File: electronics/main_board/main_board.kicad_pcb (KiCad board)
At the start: 6 copper layers, 50 x 47 mm, 95 parts, among them CN1 DB141R-2.54-2P, CN3 KF202-5.0-3P, U1 HUSB238A-BB001-QN16R, U10 TJA1051TK/3, U11 NTTFS5C454NL, U13 NTTFS5C454NL, U14 NTTFS5C454NL, U15 NTTFS5C454NL, U16 NTTFS5C454NL, U17 NTTFS5C454NL, U18 TJA1051TK/3, U2 LMR51420YDD, U3 TPS62933DRL, U6 ESP32-S3-WROOM-1, U7 STM32G474VEH6, U8 DRV8323SRTA, U9 AFD01-S35FCA-00

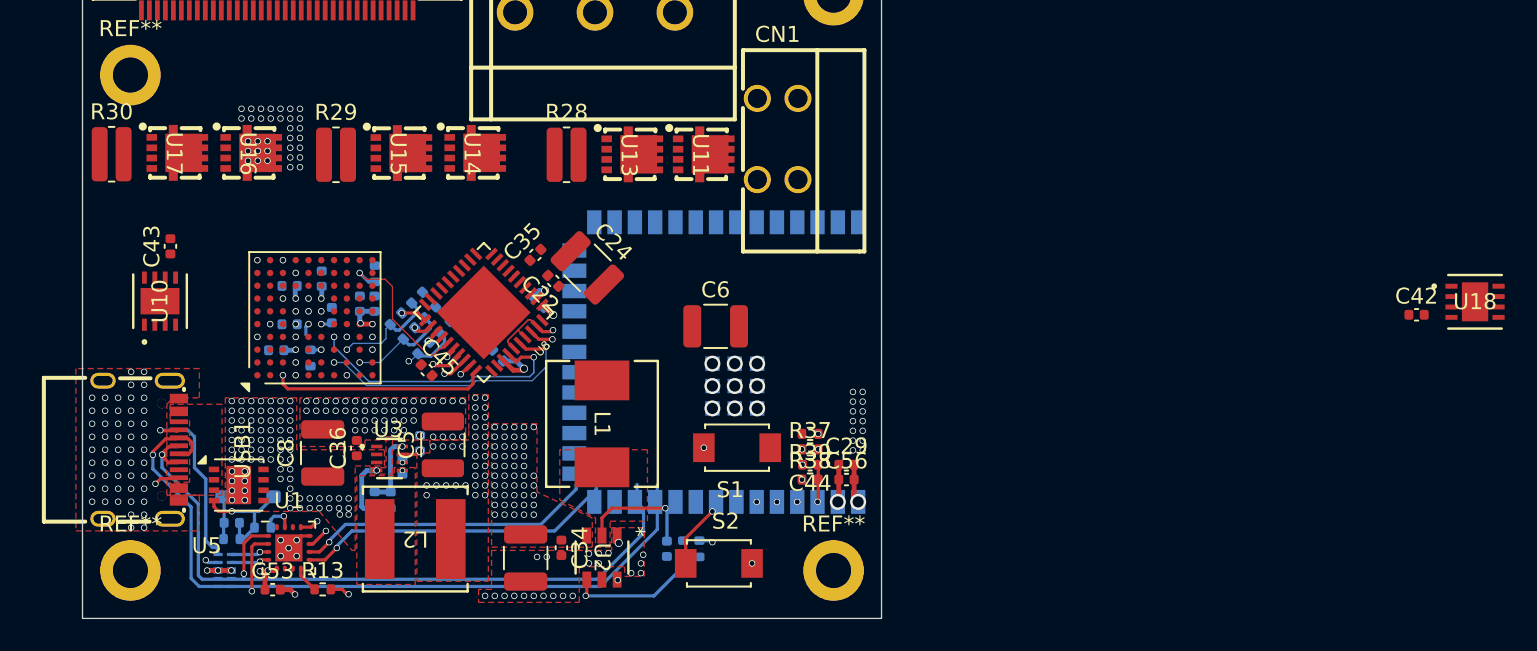
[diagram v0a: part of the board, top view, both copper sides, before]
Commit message: fix
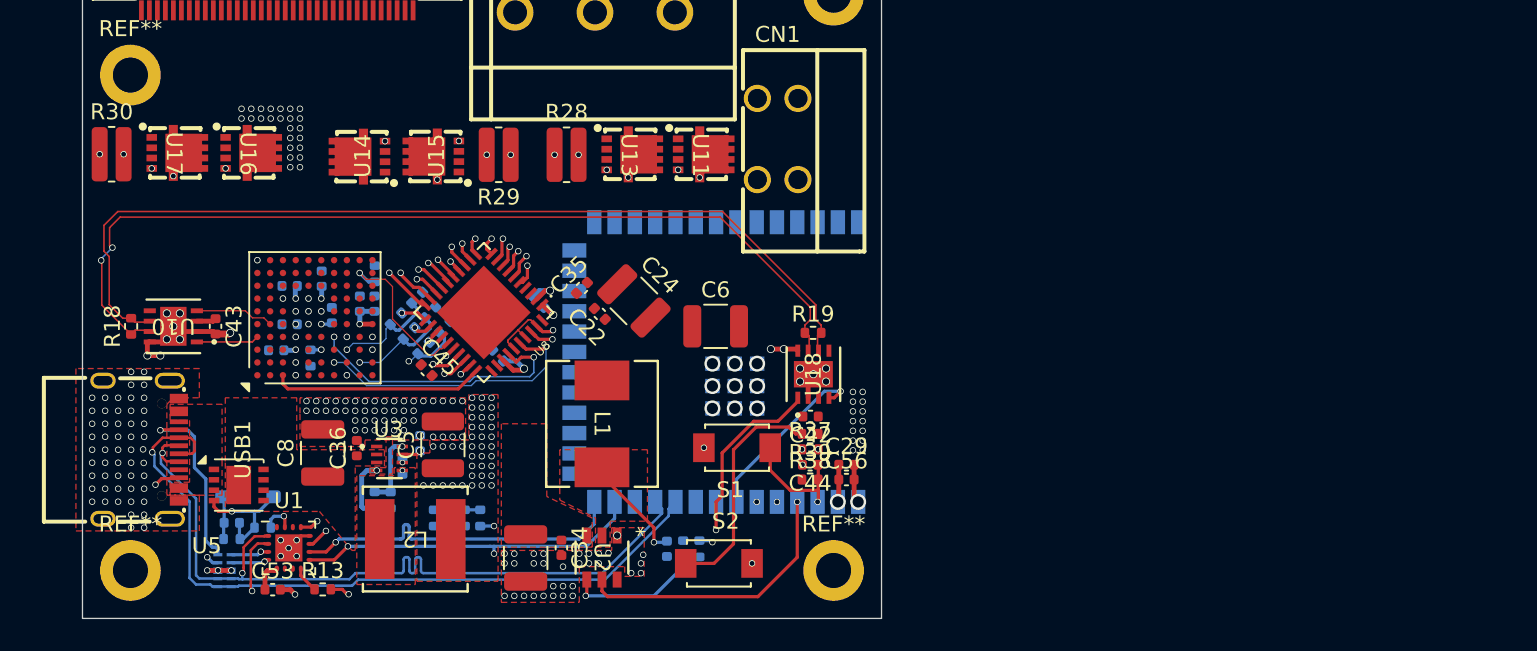
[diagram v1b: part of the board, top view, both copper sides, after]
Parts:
- added R18: 120, Resistor_SMD:R_0402_1005Metric, F.Cu at (117.0, 96.7)
- added R19: 120, Resistor_SMD:R_0402_1005Metric, F.Cu at (159.7, 97.1)
- added R40: 10k, Resistor_SMD:R_0402_1005Metric, B.Cu at (137.9, 108.7)
- added R41: 10k, Resistor_SMD:R_0402_1005Metric, B.Cu at (136.0, 108.7)
- added R42: 10k, Resistor_SMD:R_0402_1005Metric, B.Cu at (138.9, 108.7)
- added R43: 10k, Resistor_SMD:R_0402_1005Metric, B.Cu at (137.0, 108.7)
- moved U18 41.6 mm to (159.7, 99.7), turned to 90 degrees
- moved C42 38.4 mm to (159.6, 102.4), turned to 180 degrees
- moved R29 10.2 mm to (140.0, 86.0), turned to 180 degrees
- moved U14 6.85 mm to (131.5, 86.1), turned to 90 degrees
- moved C43 5.75 mm to (122.3, 96.7), turned to -90 degrees
- moved C35 3.57 mm to (145.3, 94.3)
- moved C22 3.57 mm to (146.4, 95.9)
- moved C24 3.57 mm to (148.5, 95.1)
- moved U15 2.40 mm to (136.2, 86.0), turned to 90 degrees
- moved U10 1.78 mm to (119.7, 96.7), turned to 180 degrees
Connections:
- net /CANH renamed /CAN_P
- net /CANL renamed /CAN_N
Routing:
- net /CAN_N: track 0.00 -> 58.6 mm
- net /CAN_P: track 0.00 -> 58.4 mm, vias 0 -> 2
- net GND: track 12.7 -> 63.9 mm, vias 155 -> 186
- net /Motor/Gate Driver/H_BRIDGE_SPC: track 0.00 -> 25.7 mm, vias 0 -> 2
- net /Motor/Gate Driver/H_BRIDGE_GLC: track 0.00 -> 23.1 mm, vias 0 -> 2
- net /Motor/Gate Driver/H_BRIDGE_SHC: track 0.00 -> 21.0 mm, vias 0 -> 2
- net /Motor/Gate Driver/H_BRIDGE_GHC: track 0.18 -> 17.7 mm, vias 0 -> 2
- net /MCU/EN_12V: track 4.92 -> 22.3 mm
- net VBUS: track 0.00 -> 15.2 mm, vias 133 -> 2
- net /Motor/Gate Driver/H_BRIDGE_GHA: track 0.37 -> 14.3 mm, vias 0 -> 2
- net /CAN Transceiver1/CAN_TX: track 0.00 -> 11.3 mm, vias 0 -> 1
- net /CAN Transceiver1/CAN_RX: track 0.00 -> 11.1 mm, vias 0 -> 1
- net /Motor/Gate Driver/H_BRIDGE_SHA: track 0.00 -> 10.7 mm, vias 0 -> 2
- net Net-(U6-IO0): track 3.94 -> 14.4 mm, vias 1 -> 0
- net /Motor/Gate Driver/H_BRIDGE_GHB: track 0.00 -> 10.2 mm, vias 0 -> 2
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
